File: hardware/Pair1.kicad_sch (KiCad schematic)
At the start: 11 parts, among them J12 Conn_01x02, J4 Conn_01x02

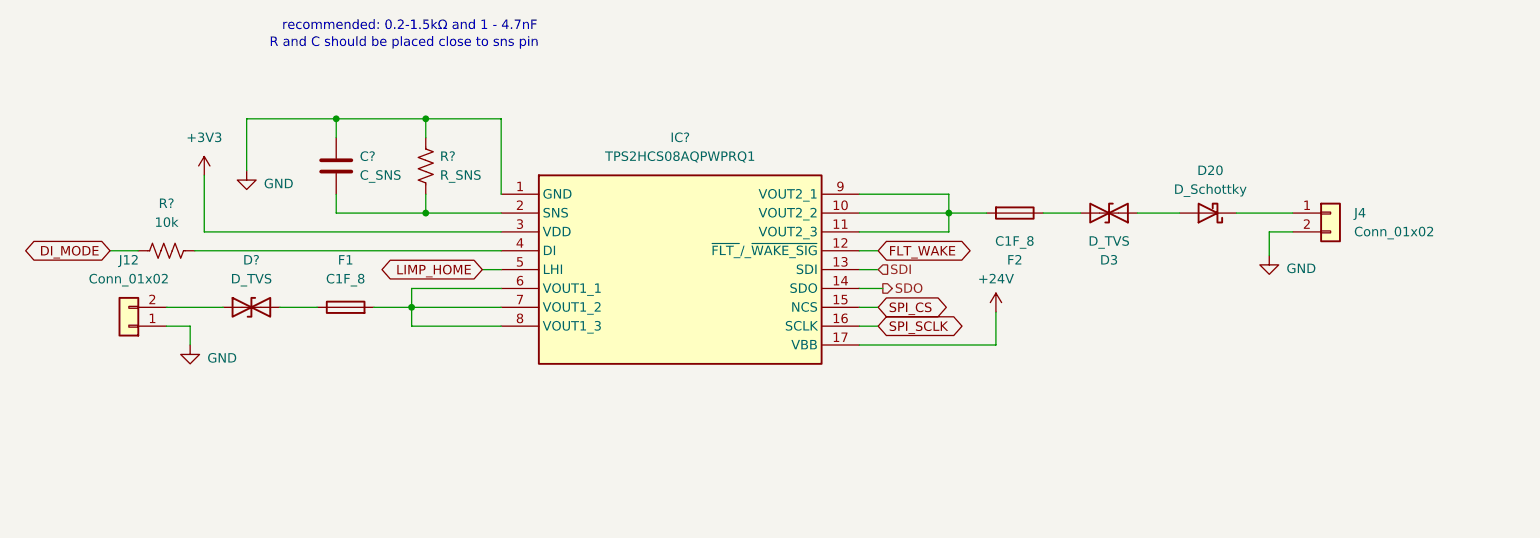
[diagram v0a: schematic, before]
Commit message: aesthetic added
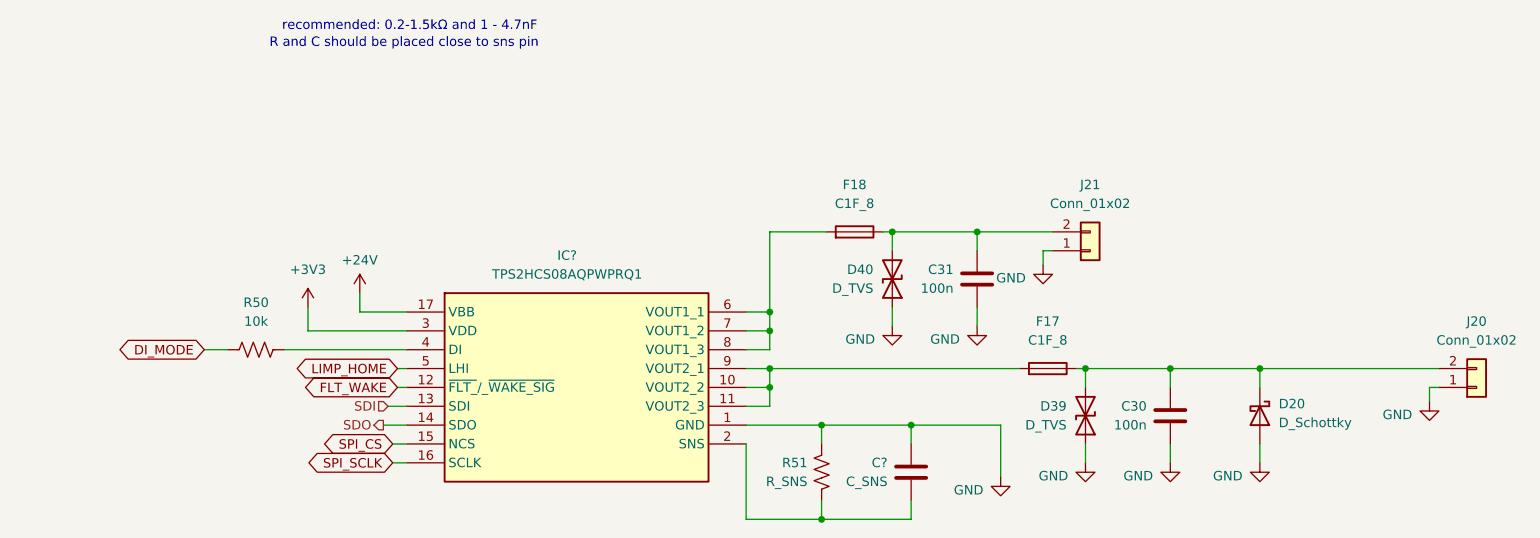
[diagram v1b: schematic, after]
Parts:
- removed D3, D?: D_TVS, symbol Device:D_TVS
- removed F1, F2: C1F_8, Fuse:Fuse_1206_3216Metric, symbol PowerDistributionUnitLib:C1F_8
- removed J12, J4: Conn_01x02, symbol Connector_Generic:Conn_01x02
- removed R?: 10k, symbol Device:R_US
- removed R?: R_SNS, symbol Device:R_US
- added C30, C31: 100n, symbol Device:C
- added D39, D40: D_TVS, symbol Device:D_TVS
- added F17, F18: C1F_8, Fuse:Fuse_1206_3216Metric, symbol PowerDistributionUnitLib:C1F_8
- added J20, J21: Conn_01x02, symbol Connector_Generic:Conn_01x02
- added R50: 10k, symbol Device:R_US
- added R51: R_SNS, symbol Device:R_US
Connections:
- net DI_MODE: now also R50.2
- net GND: now also D20.2 (A), C30.1, C31.1, D39.1 (A1), D40.1 (A1), J20.1 (Pin_1), J21.1 (Pin_1), R51.2
- net at IC?.10 (VOUT2_2), IC?.11 (VOUT2_3), IC?.9 (VOUT2_1): now also F17.2
- net at C?.1, IC?.2 (SNS): now also R51.1
- net at IC?.4 (DI): now also R50.1
- net at IC?.6 (VOUT1_1), IC?.7 (VOUT1_2), IC?.8 (VOUT1_3): now also F18.2
- net at D20.1 (K): now also C30.2, D39.2 (A2), F17.1, J20.2 (Pin_2)
- new net: C31.2, D40.2 (A2), F18.1, J21.2 (Pin_2)
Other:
- moved on the sheet: C?, IC?
